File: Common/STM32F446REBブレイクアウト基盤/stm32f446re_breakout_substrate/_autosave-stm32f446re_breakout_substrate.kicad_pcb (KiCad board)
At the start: 2 copper layers, 83.8 x 114.2 mm, 88 parts, among them J1 Conn_01x07_Socket, J10 Conn_01x03_Socket, J11 Conn_01x03_Socket, J12 Conn_01x03_Socket, J13 Conn_01x03_Socket, J14 Conn_01x03_Socket, J15 Conn_01x03_Socket, J16 Conn_01x03_Socket, J17 Conn_01x03_Socket, J18 Conn_01x10_Socket, J19 Conn_01x10_Socket, J2 Conn_01x04_Socket, J20 Conn_01x03_Socket, J21 Conn_01x10_Socket, J22 Conn_01x02_Socket, J23 Conn_01x03_Socket, J24 J1_B, J25 J2_B, J26 J3_B, J27 J1_A, J28 J2_A, J29 J3_A, J3 Conn_01x04_Socket, J30 J4_B, J31 J5_B, J32 J4_A, J33 J5_A, J34 J6_B, J35 J7_B, J36 J6_A, J37 J7_A, J38 J9_B, J39 J8_B, J4 Conn_01x04_Socket, J40 J8_A, J41 J9_A, J42 J10_B, J43 J10_A, J44 J11_B, J45 J11_A, J46 J12_B, J47 J12_A, J48 J13_B, J49 J13_A, J5 Conn_01x04_Socket, J50 J14_B, J51 J14_A, J52 J16_B, J53 J15_B, J54 J15_A, J55 J16_A, J56 J17_B, J57 J17_A, J58 J18_A, J59 J19_A, J6 Conn_01x04_Socket, J60 J20_A, J61 J20_A, J62 J19_A, J63 J18_A, J64 Conn_01x15_Socket, J65 Conn_01x15_Socket, J66 J21_A, J67 J21_B, J68 J22_B, J69 J22_A, J7 Conn_01x04_Socket, J70 J23_B, J71 J23_A, J8 Conn_01x04_Socket, J9 Conn_01x03_Socket, SW1 SW_Push, SW2 SW_Push

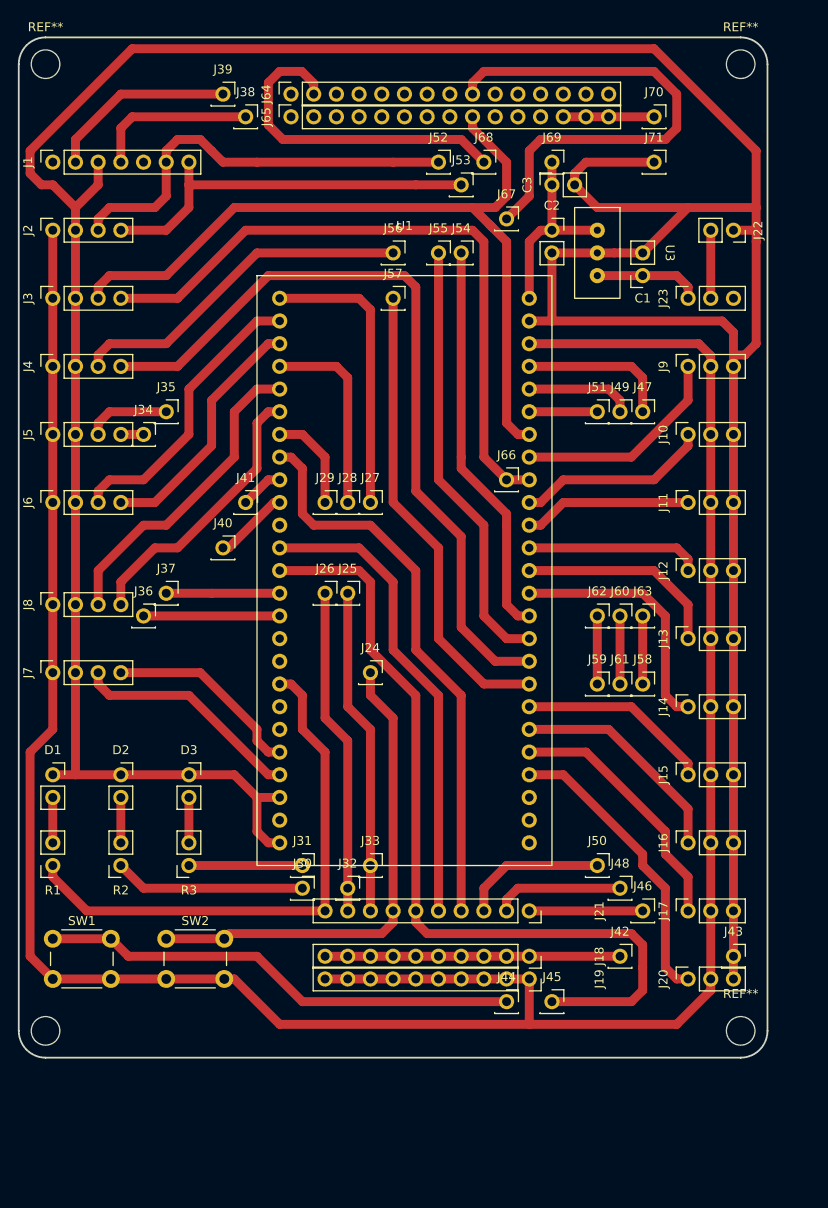
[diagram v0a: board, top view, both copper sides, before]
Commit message: e
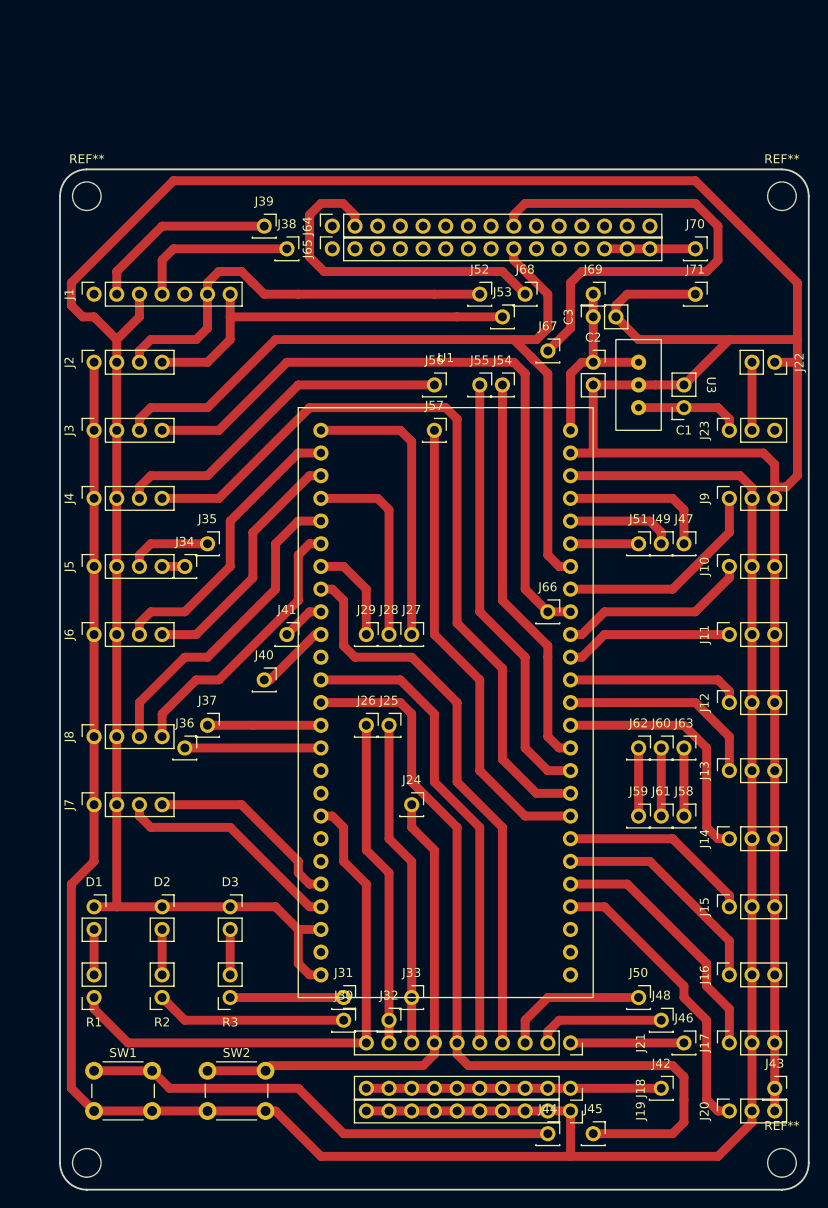
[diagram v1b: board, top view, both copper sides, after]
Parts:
- moved D1 15.5 mm to (4.62, 83.4)
- moved D2 15.5 mm to (12.2, 83.4)
- moved D3 15.5 mm to (19.9, 83.4)
- moved J19 15.5 mm to (58.0, 106.2)
- moved J21 15.5 mm to (58.0, 98.6)
- moved J25 15.5 mm to (37.6, 63.0)
- moved J32 15.5 mm to (37.6, 96.1)
- moved J33 15.5 mm to (40.2, 93.5)
- moved J36 15.5 mm to (14.8, 65.6)
- moved J37 15.5 mm to (17.3, 63.0)
- moved J4 15.5 mm to (4.62, 37.6)
- moved J40 15.5 mm to (23.7, 58.0)
- moved J48 15.5 mm to (68.1, 96.1)
- moved J49 15.5 mm to (68.1, 42.7)
- moved J50 15.5 mm to (65.6, 93.5)
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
